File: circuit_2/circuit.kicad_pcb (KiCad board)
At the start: 2 copper layers, 64 parts, among them U1 MIC5219BM5_SOT23-5

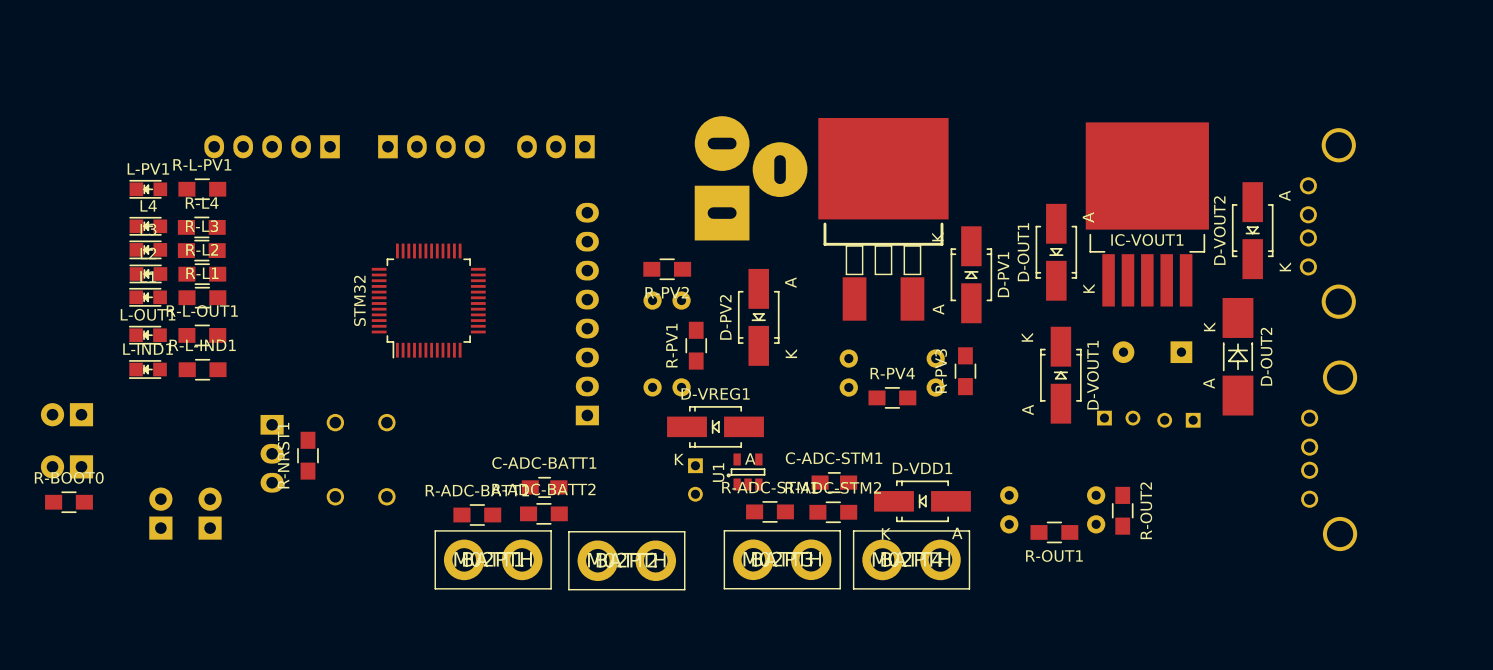
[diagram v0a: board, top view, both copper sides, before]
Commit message: circuit 2
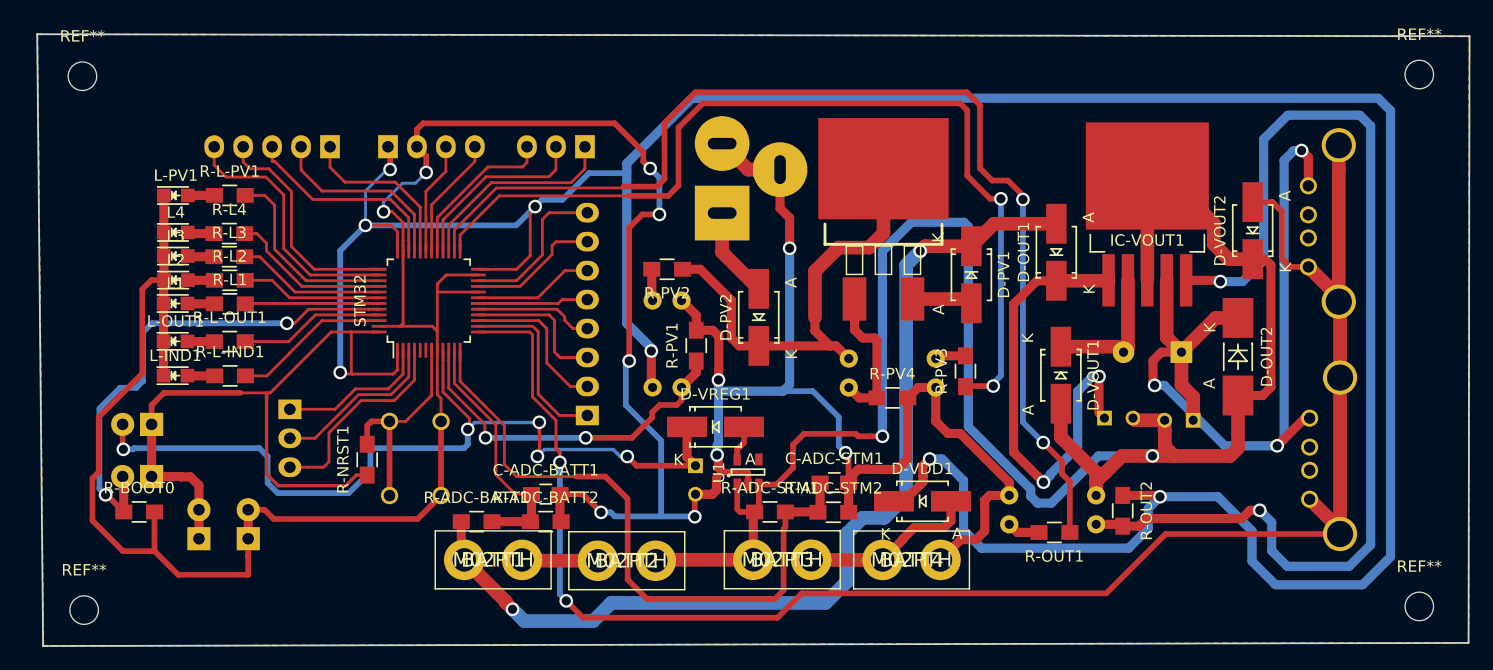
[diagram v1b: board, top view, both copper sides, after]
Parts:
- added REF**: MountingHole_2-5mm, Mounting_Holes:MountingHole_2-5mm, F.Cu at (88.8, 128.7)
- added REF**: MountingHole_2-5mm, Mounting_Holes:MountingHole_2-5mm, F.Cu at (88.6, 81.9)
- added REF**: MountingHole_2-5mm, Mounting_Holes:MountingHole_2-5mm, F.Cu at (205.9, 81.8)
- added REF**: MountingHole_2-5mm, Mounting_Holes:MountingHole_2-5mm, F.Cu at (205.9, 128.4)
- moved P-BOOT1 6.21 mm to (94.7, 117.0)
- moved P-VDD-3V3 6.21 mm to (94.7, 112.4)
- moved R-BOOT0 6.21 mm to (93.6, 120.1)
- moved R-NRST1 5.20 mm to (113.6, 115.5)
- moved SW-NRST1 4.75 mm to (117.8, 115.4)
- moved P-GND1 3.47 mm to (103.2, 122.5)
- moved P-VDD1 3.47 mm to (98.9, 122.5)
- moved L-IND1 2.47 mm to (96.8, 108.2)
- moved L-PV1 2.47 mm to (96.8, 92.4)
- moved L1 2.47 mm to (96.8, 101.8)
- moved L2 2.47 mm to (96.8, 99.8)
- moved L3 2.47 mm to (96.8, 97.7)
- moved L4 2.47 mm to (96.8, 95.6)
- moved R-L-OUT1 2.47 mm to (101.6, 105.2)
- moved R-L-PV1 2.47 mm to (101.6, 92.4)
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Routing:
- net VDD: track 0.00 -> 319.9 mm, vias 0 -> 7
- net GND: track 0.00 -> 317.9 mm, vias 0 -> 11
- net +6V: track 0.00 -> 168.7 mm, vias 0 -> 2
- net /ADC_OUT: track 0.00 -> 153.8 mm, vias 0 -> 2
- net /CON_OUT: track 0.00 -> 97.8 mm, vias 0 -> 2
- net Net-(IC-VOUT1-Pad5): track 0.00 -> 94.6 mm, vias 0 -> 2
- net +15V: track 0.00 -> 86.4 mm, vias 0 -> 2
- net /CON_PV: track 0.00 -> 82.6 mm, vias 0 -> 2
- net +3V3: track 0.00 -> 75.6 mm, vias 0 -> 5
- net Net-(C_VOUT1-Pad1): track 0.00 -> 71.8 mm, vias 0 -> 3
- net /ADC_STM: track 0.00 -> 57.9 mm
- net /BOOT0: track 0.00 -> 43.9 mm, vias 0 -> 2
- net Net-(C-OUT1-Pad1): track 0.00 -> 41.4 mm, vias 0 -> 2
- net +24V: track 0.00 -> 39.9 mm
- net /IND_PV_WKUP: track 0.00 -> 31.9 mm, vias 0 -> 2
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- added copper zone on B.Cu, net (none)
- added copper zone on F.Cu, net (none)
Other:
- board outline added: 125.6 x 53.6 mm
- net class Default: clearance 0.2 -> 0.1; via_dia 0.6 -> 1.2; via_drill 0.4 -> 0.8
- rule trace_clearance: 0.2 -> 0.1
